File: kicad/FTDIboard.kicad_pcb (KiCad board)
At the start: 4 copper layers, 50 x 75 mm, 84 parts, among them J1 USB_C_Receptacle_USB2.0_14P, J4 Conn_01x07, J5 Conn_01x04, Q1 AO3401A, Q2 BC817, Q3 BC817, SW1 SW_SPDT_321, U1 USBLC6-2SC6, U2 TLV75733PDBV, U3 FT232RL, U4 ULN2003, U5 ULN2003

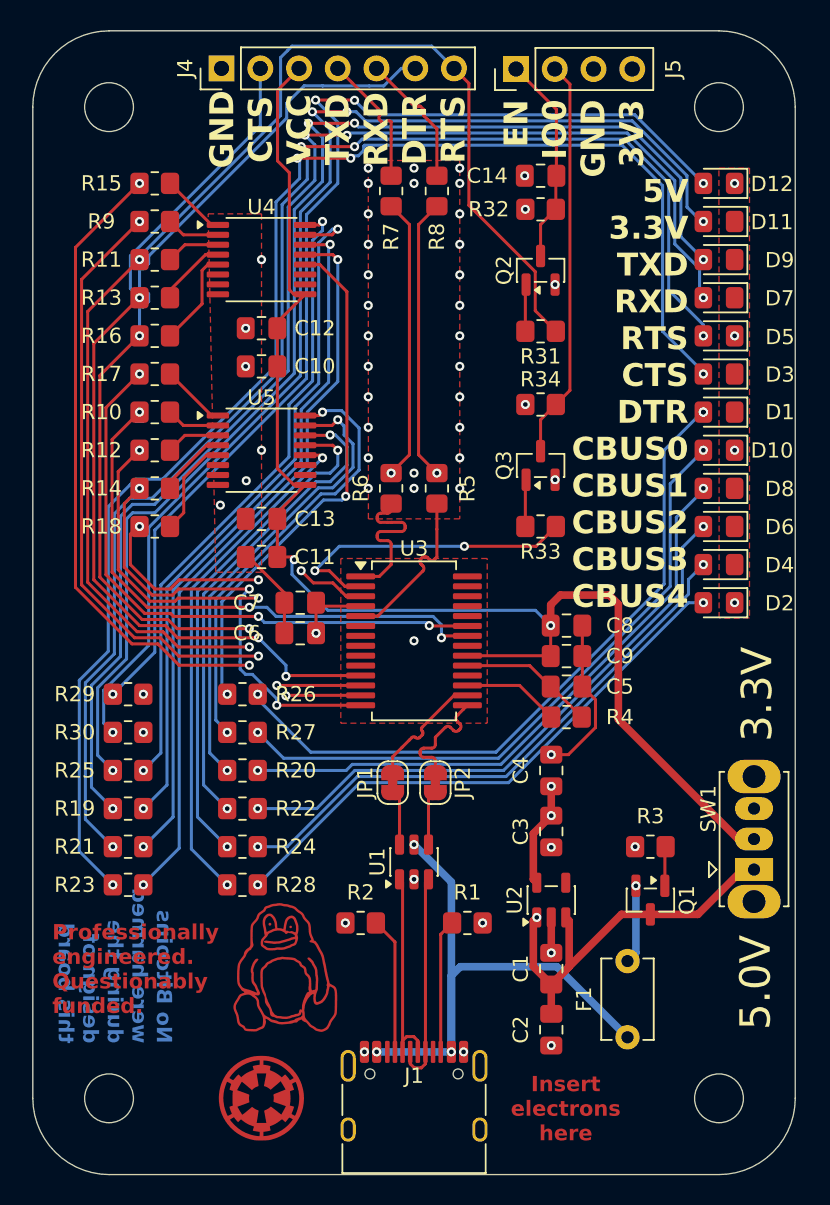
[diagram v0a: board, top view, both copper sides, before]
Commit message: v1.1
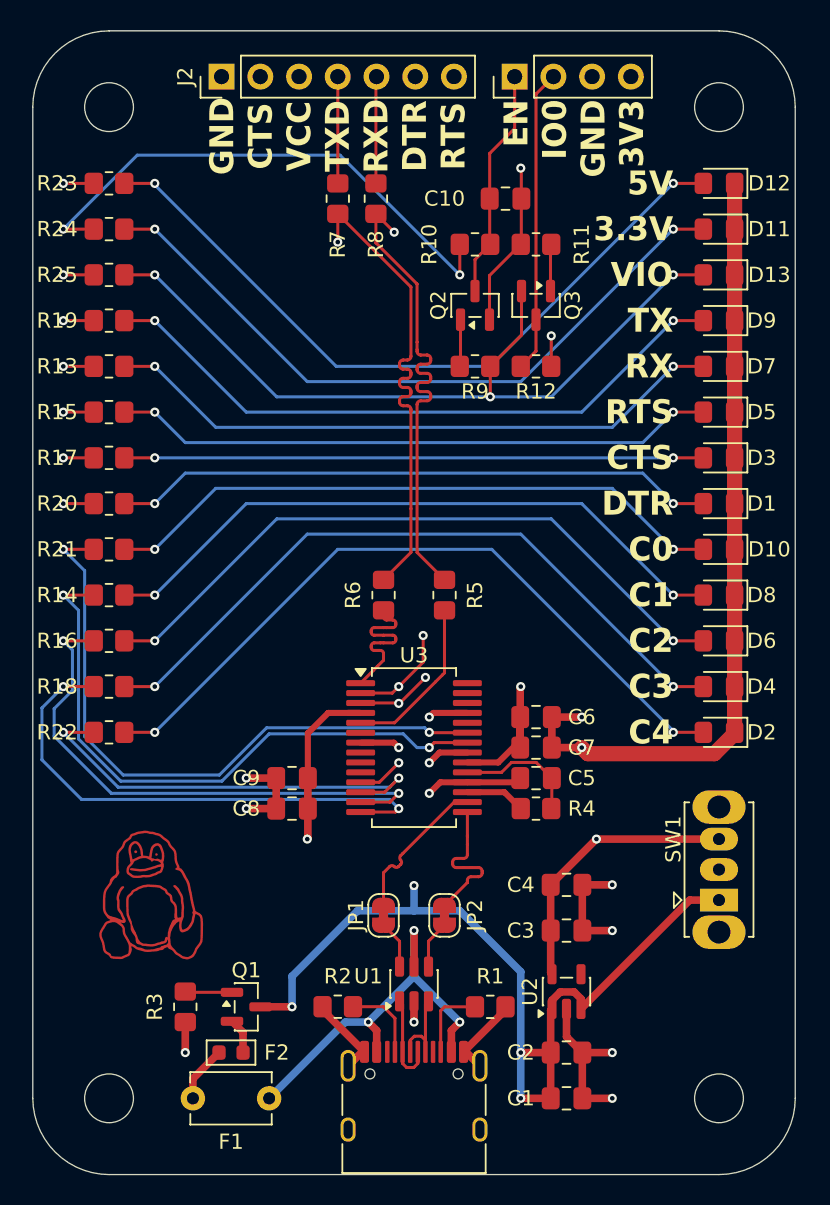
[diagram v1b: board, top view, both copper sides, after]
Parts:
- removed C11, C14: 100nF, Capacitor_SMD:C_0805_2012Metric_Pad1.18x1.45mm_HandSolder
- removed C12, C13: 10uF, Capacitor_SMD:C_0805_2012Metric_Pad1.18x1.45mm_HandSolder
- removed the G*** at (30.0, 85.0) (x2)
- removed J4: Conn_01x07, Connector_PinHeader_2.54mm:PinHeader_1x07_P2.54mm_Vertical
- removed J5: Conn_01x04, Connector_PinHeader_2.54mm:PinHeader_1x04_P2.54mm_Vertical
- removed R26, R27, R28, R29, R30, R32, R34: 10k, Resistor_SMD:R_0805_2012Metric_Pad1.20x1.40mm_HandSolder
- removed R31, R33: 1k, Resistor_SMD:R_0805_2012Metric_Pad1.20x1.40mm_HandSolder
- removed U4, U5: ULN2003, Package_SO:TSSOP-16_4.4x5mm_P0.65mm
- added D13: LED, LED_SMD:LED_0805_2012Metric_Pad1.15x1.40mm_HandSolder, F.Cu at (60.0, 31.0)
- added F2: 2.5A, Fuse_US_Handsoldering_AKL:Fuse_0603_1608Metric, F.Cu at (28.0, 82.0)
- added J2: Conn_01x07, Connector_PinHeader_2.54mm:PinHeader_1x07_P2.54mm_Vertical, F.Cu at (27.4, 18.0)
- added J3: Conn_01x04, Connector_PinHeader_2.54mm:PinHeader_1x04_P2.54mm_Vertical, F.Cu at (46.6, 18.0)
- R11, R9: value 10k -> 1k
- moved R23 46.0 mm to (20.0, 25.0), turned to 0 degrees
- moved R24 41.4 mm to (20.0, 28.0)
- moved R25 32.5 mm to (20.0, 31.0), turned to 0 degrees
- moved R3 32.3 mm to (25.0, 79.0), turned to -90 degrees
- moved R19 32.0 mm to (20.0, 34.0), turned to 0 degrees
- moved Q1 27.4 mm to (29.0, 79.0), turned to 0 degrees
- moved R12 25.6 mm to (48.0, 37.0), turned to 180 degrees
- moved R11 25.0 mm to (48.0, 29.0)
- moved F1 23.8 mm to (30.5, 85.0), turned to 180 degrees
- moved R10 23.7 mm to (44.0, 29.0)
- moved R9 23.0 mm to (44.0, 37.0), turned to 180 degrees
- moved C8 21.6 mm to (32.0, 66.0), turned to 180 degrees
- moved R16 20.2 mm to (20.0, 55.0)
- moved C9 19.7 mm to (32.0, 64.0), turned to 180 degrees
- moved R20 19.6 mm to (20.0, 46.0)
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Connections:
- C10 pad 1: /LED_INDICATORS/VIO -> ESP_EN
- C10 pad 2: GND -> /ESP_AUTO_RST/DTR_N
- C6 pad 1: /LED_INDICATORS/5V_USB -> /LED_INDICATORS/VIO
- C7 pad 1: /LED_INDICATORS/5V_USB -> /LED_INDICATORS/VIO
- F1 pad 2: VBUS_PROTECTED -> Net-(F1-Pad2)
- Q2 pad 2: GND -> /ESP_AUTO_RST/DTR_N
- Q3 pad 2: GND -> /ESP_AUTO_RST/RTS_N
- R10 pad 1: /LED_INDICATORS/CBUS1 -> /3.3V
- R10 pad 2: Net-(U5-I2) -> ESP_EN
- R11 pad 1: /ESP_AUTO_RST/RTS_N -> /ESP_AUTO_RST/DTR_N
- R11 pad 2: Net-(U4-I3) -> Net-(Q3-B)
- R12 pad 1: /LED_INDICATORS/CBUS2 -> /3.3V
- R12 pad 2: Net-(U5-I3) -> ESP_IO0
- R13 pad 1: /LED_INDICATORS/CTS -> /LED_INDICATORS/RXD_IN
- R13 pad 2: Net-(U4-I4) -> Net-(D7-A)
- R14 pad 1: /LED_INDICATORS/CBUS3 -> /LED_INDICATORS/CBUS1
- R14 pad 2: Net-(U5-I4) -> Net-(D8-A)
- R15 pad 1: /LED_INDICATORS/TXD_OUT -> /ESP_AUTO_RST/RTS_N
- R15 pad 2: Net-(U4-I1) -> Net-(D5-A)
- R16 pad 1: /ESP_AUTO_RST/DTR_N -> /LED_INDICATORS/CBUS2
- R16 pad 2: Net-(U4-I5) -> Net-(D6-A)
- R17 pad 1: /LED_INDICATORS/CBUS0 -> /LED_INDICATORS/CTS
- R17 pad 2: Net-(U5-I1) -> Net-(D3-A)
- R18 pad 1: /LED_INDICATORS/CBUS4 -> /LED_INDICATORS/CBUS3
- R18 pad 2: Net-(U5-I5) -> Net-(D4-A)
- R19 pad 1: Net-(U4-O2) -> /LED_INDICATORS/TXD_OUT
- R19 pad 2: Net-(D7-A) -> Net-(D9-A)
- R20 pad 1: Net-(U5-O2) -> /ESP_AUTO_RST/DTR_N
- R20 pad 2: Net-(D8-A) -> Net-(D1-A)
- R21 pad 1: Net-(U4-O3) -> /LED_INDICATORS/CBUS0
- R21 pad 2: Net-(D5-A) -> Net-(D10-A)
- R22 pad 1: Net-(U5-O3) -> /LED_INDICATORS/CBUS4
- R22 pad 2: Net-(D6-A) -> Net-(D2-A)
- R23 pad 1: Net-(U4-O4) -> /LED_INDICATORS/5V_USB
- R23 pad 2: Net-(D3-A) -> Net-(D12-A)
- R24 pad 1: Net-(U5-O4) -> /3.3V
- R24 pad 2: Net-(D4-A) -> Net-(D11-A)
- R25 pad 1: Net-(U4-O1) -> /LED_INDICATORS/VIO
- R25 pad 2: Net-(D9-A) -> Net-(D13-A)
- R9 pad 1: /LED_INDICATORS/RXD_IN -> /ESP_AUTO_RST/RTS_N
- R9 pad 2: Net-(U4-I2) -> Net-(Q2-B)
- U3 pad 4: /LED_INDICATORS/5V_USB -> /LED_INDICATORS/VIO
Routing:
- net /3.3V: track 8.04 -> 116.9 mm, vias 5 -> 4
- net GND: track 19.2 -> 104.6 mm, vias 52 -> 14
- net /LED_INDICATORS/VIO: track 90.6 -> 22.6 mm, vias 2 -> 3
- net Net-(D3-A): track 94.7 -> 38.0 mm, vias 4 -> 2
- net /LED_INDICATORS/5V_USB: track 71.4 -> 122.8 mm, vias 3 -> 5
- net Net-(D5-A): track 90.7 -> 39.6 mm, vias 4 -> 2
- net Net-(U4-O4): track 48.6 -> 0.00 mm, vias 2 -> 0
- net Net-(U4-O3): track 46.2 -> 0.00 mm, vias 2 -> 0
- net Net-(U4-O2): track 45.8 -> 0.00 mm, vias 2 -> 0
- net Net-(D7-A): track 86.0 -> 41.3 mm, vias 4 -> 2
- net Net-(D13-A): track 0.00 -> 44.6 mm, vias 0 -> 2
- net Net-(U4-O1): track 42.1 -> 0.00 mm, vias 2 -> 0
- net Net-(D9-A): track 82.1 -> 42.9 mm, vias 4 -> 2
- net /LED_INDICATORS/CTS: track 59.1 -> 93.6 mm, vias 3 -> 2
- net Net-(U4-O5): track 34.2 -> 0.00 mm, vias 2 -> 0
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- added copper zone on In2.Cu, net /LED_INDICATORS/VIO
- added copper zone on In1.Cu, net GND
- removed copper zone on In1.Cu, net /3.3V
- removed copper zone on F.Cu, net GND
- removed copper zone on In2.Cu, net GND
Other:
- board text added: "5V"
- board text added: "C0"
- board text added: "C1"
- board text added: "C2"
- board text added: "C3"
- board text added: "C4"
- board text added: "CTS"
- board text added: "DTR"
- board text added: "RTS"
- board text added: "RX"
- board text added: "TX"
- board text added: "VIO"
- board text removed: "200 OK - MOON REACHABLE"
- board text removed: "5.0V"
- board text removed: "5V 3.3V TXD RXD RTS CTS DTR CBUS0 CBUS1 CBUS2 CBUS3 CBUS4"
- board text removed: "Insert electrons here"
- board text removed: "No Bitcoins were harmed during the design of this board"
- board text removed: "Professionally engineered. Questionably funded."
- board text removed: "{dblquote}I have two Microsoft Outlooks and neither one of those are working.{dblquote} - Reid Wiseman, Artemis II"
